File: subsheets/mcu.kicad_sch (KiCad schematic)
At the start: 25 parts, among them J2 Conn_01x05, U5 LoRa-E5

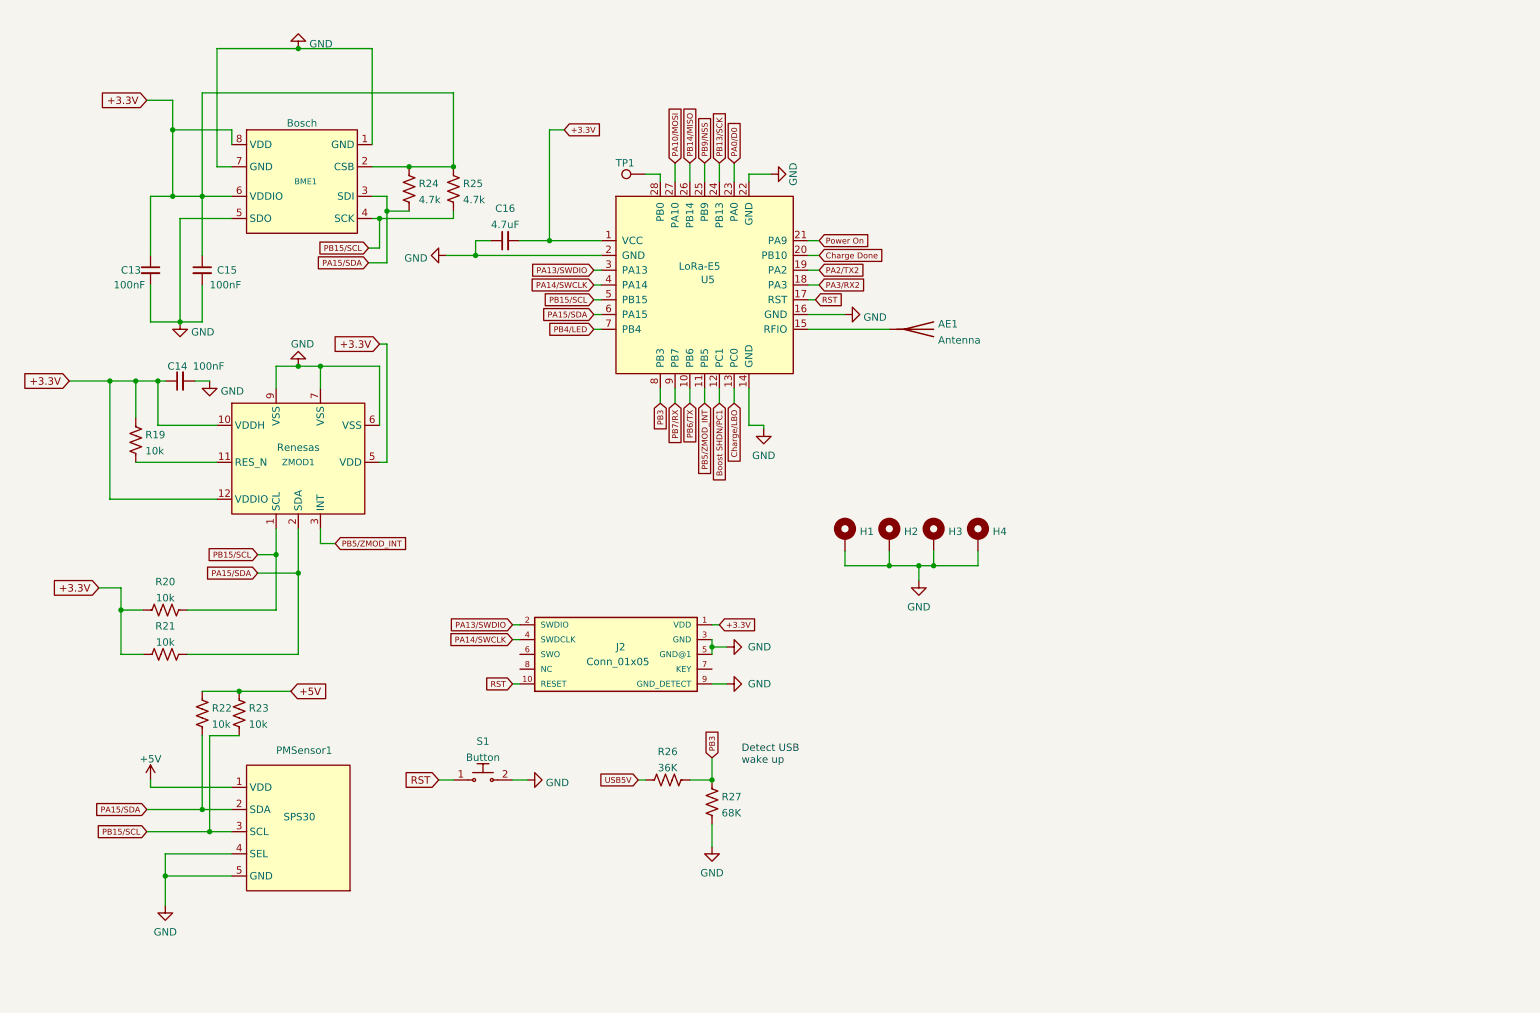
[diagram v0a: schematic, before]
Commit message: Final Schematic
-
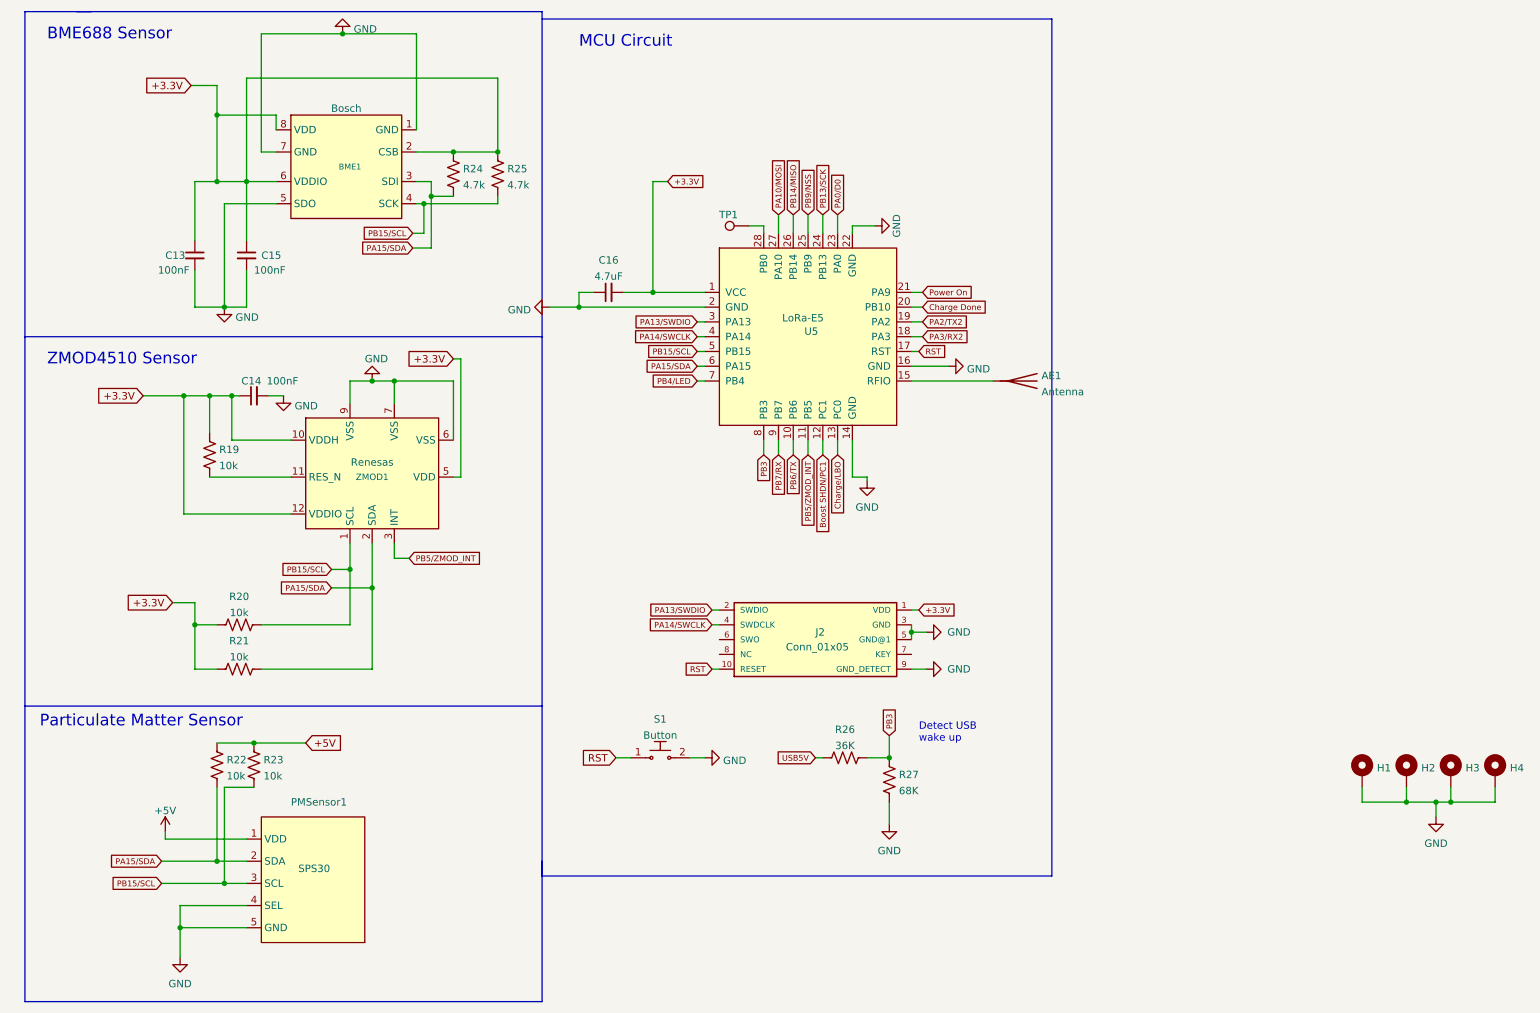
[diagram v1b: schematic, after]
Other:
- note added: "BME688 Sensor"
- note added: "MCU Circuit"
- note added: "Particulate Matter Sensor"
- note added: "ZMOD4510 Sensor"
- moved on the sheet: AE1, BME1, C13, C14, C15, C16, H1, H2, H3, H4, J2, PMSensor1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
